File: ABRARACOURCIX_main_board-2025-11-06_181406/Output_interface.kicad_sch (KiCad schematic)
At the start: 11 parts, among them J10 Conn_01x03_Socket, J11 Conn_01x03_Socket, J6 Conn_01x03_Socket, J8 Conn_01x03_Socket, J9 Conn_01x03_Socket, Q1 MMBT3904

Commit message: Placement des composantes 95%
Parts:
- C27: footprint Capacitor_SMD:C_1206_3216Metric_Pad1.33x1.80mm_HandSolder -> Librairie_footprint:CAP_R533W520050P0K_KEM
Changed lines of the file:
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@@
 			)
 		)
-		(property "Footprint" "Capacitor_SMD:C_1206_3216Metric_Pad1.33x1.80mm_HandSolder"
+		(property "Footprint" "Librairie_footprint:CAP_R533W520050P0K_KEM"
 			(at 45.4152 85.09 0)
 			(effects

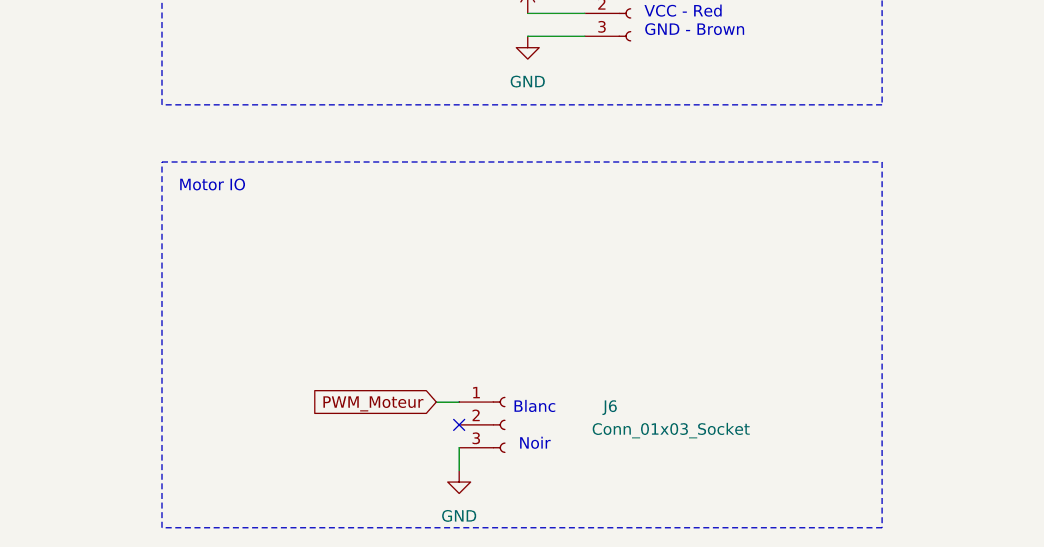
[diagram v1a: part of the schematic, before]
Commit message: Documentation de composantes
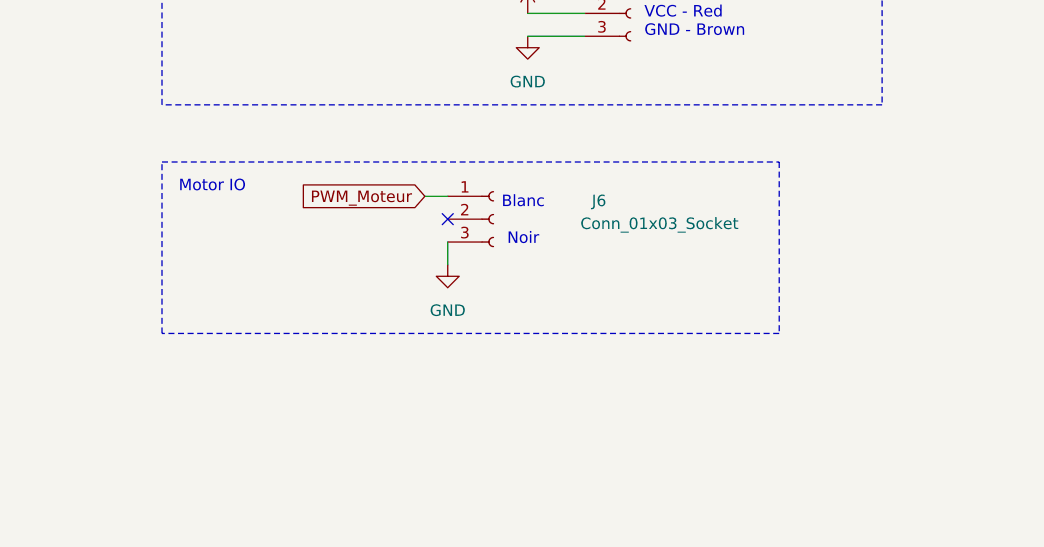
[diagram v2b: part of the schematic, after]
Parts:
- C27: footprint Librairie_footprint:CAP_R533W520050P0K_KEM -> Librairie_footprint:CAP_MU_15750_RUB-L
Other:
- moved on the sheet: J6
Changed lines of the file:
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@@
 	(rectangle
 		(start 36.83 137.16)
-		(end 116.84 177.8)
+		(end 105.41 156.21)
 		(stroke
 			(width 0)
@@
 	(text "Blanc\n\nNoir\n"
 		(exclude_from_sim no)
-		(at 78.232 166.624 0)
+		(at 76.962 143.764 0)
 		(effects
 			(font
@@
 	)
 	(no_connect
-		(at 69.85 166.37)
+		(at 68.58 143.51)
 	)
 	(wire
@@
 	(wire
 		(pts
-			(xy 67.31 163.83) (xy 69.85 163.83)
-		)
-		(stroke
-			(width 0)
-			(type default)
-		)
-	)
-	(wire
-		(pts
-			(xy 69.85 171.45) (xy 69.85 168.91)
+			(xy 66.04 140.97) (xy 68.58 140.97)
+		)
+		(stroke
+			(width 0)
+			(type default)
+		)
+	)
+	(wire
+		(pts
+			(xy 68.58 148.59) (xy 68.58 146.05)
 		)
 		(stroke
@@
 	(global_label "PWM_Moteur"
 		(shape input)
-		(at 67.31 163.83 180)
+		(at 66.04 140.97 180)
 		(fields_autoplaced yes)
 		(effects
@@
 		)
 		(property "Intersheetrefs" "${INTERSHEET_REFS}"
-			(at 52.8345 163.83 0)
+			(at 51.5645 140.97 0)
 			(effects
 				(font
@@
 	(symbol
 		(lib_id "Connector:Conn_01x03_Socket")
-		(at 74.93 166.37 0)
+		(at 73.66 143.51 0)
 		(unit 1)
 		(exclude_from_sim no)
@@
 		(dnp no)
 		(property "Reference" "J6"
-			(at 85.852 164.338 0)
+			(at 84.582 141.478 0)
 			(effects
 				(font
@@
 		)
 		(property "Value" "Conn_01x03_Socket"
-			(at 84.582 166.878 0)
+			(at 83.312 144.018 0)
 			(effects
 				(font
@@
 		)
 		(property "Footprint" "Connector_PinHeader_2.54mm:PinHeader_1x03_P2.54mm_Horizontal"
-			(at 74.93 166.37 0)
+			(at 73.66 143.51 0)
 			(effects
 				(font
@@
 		)
 		(property "Datasheet" "~"
-			(at 74.93 166.37 0)
+			(at 73.66 143.51 0)
 			(effects
 				(font
@@
 		)
 		(property "Description" "Generic connector, single row, 01x03, script generated"
-			(at 74.93 166.37 0)
+			(at 73.66 143.51 0)
 			(effects
 				(font
@@
 	(symbol
 		(lib_id "power:GND")
-		(at 69.85 171.45 0)
+		(at 68.58 148.59 0)
 		(unit 1)
 		(exclude_from_sim no)
@@
 		(fields_autoplaced yes)
 		(property "Reference" "#PWR046"
-			(at 69.85 177.8 0)
+			(at 68.58 154.94 0)
 			(effects
 				(font
@@
 		)
 		(property "Value" "GND"
-			(at 69.85 176.53 0)
+			(at 68.58 153.67 0)
 			(effects
 				(font
@@
 		)
 		(property "Footprint" ""
-			(at 69.85 171.45 0)
+			(at 68.58 148.59 0)
 			(effects
 				(font
@@
 		)
 		(property "Datasheet" ""
-			(at 69.85 171.45 0)
+			(at 68.58 148.59 0)
 			(effects
 				(font
@@
 		)
 		(property "Description" "Power symbol creates a global label with name \"GND\" , ground"
-			(at 69.85 171.45 0)
+			(at 68.58 148.59 0)
 			(effects
 				(font
@@
 			)
 		)
-		(property "Footprint" "Librairie_footprint:CAP_R533W520050P0K_KEM"
+		(property "Footprint" "Librairie_footprint:CAP_MU_15750_RUB-L"
 			(at 45.4152 85.09 0)
 			(effects
